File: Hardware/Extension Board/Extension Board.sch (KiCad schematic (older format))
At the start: 7 parts, among them J1 ARDUINO_DIGITAL, J2 ARDUINO_COMMS, J3 ARDUINO_ANALOG

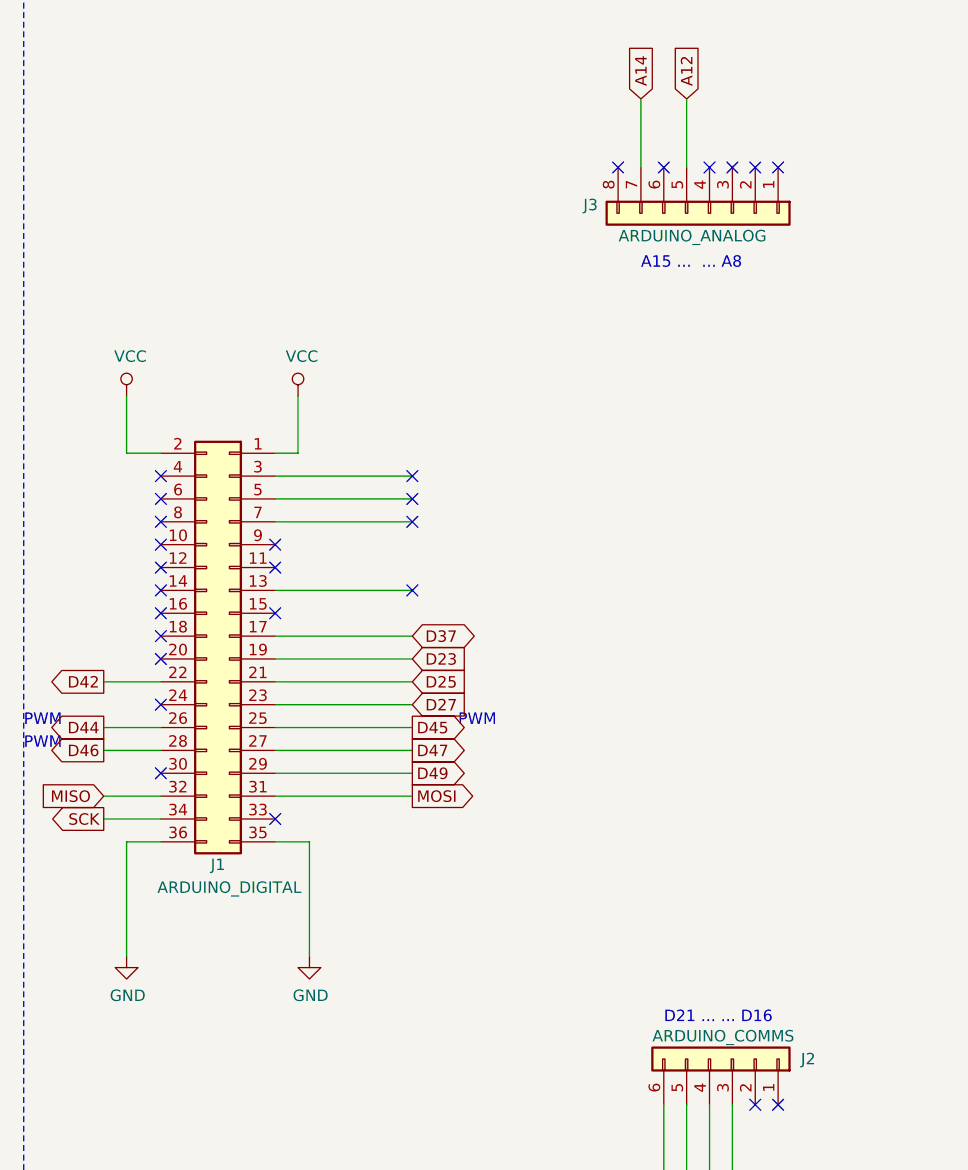
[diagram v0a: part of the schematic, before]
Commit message: début du routage
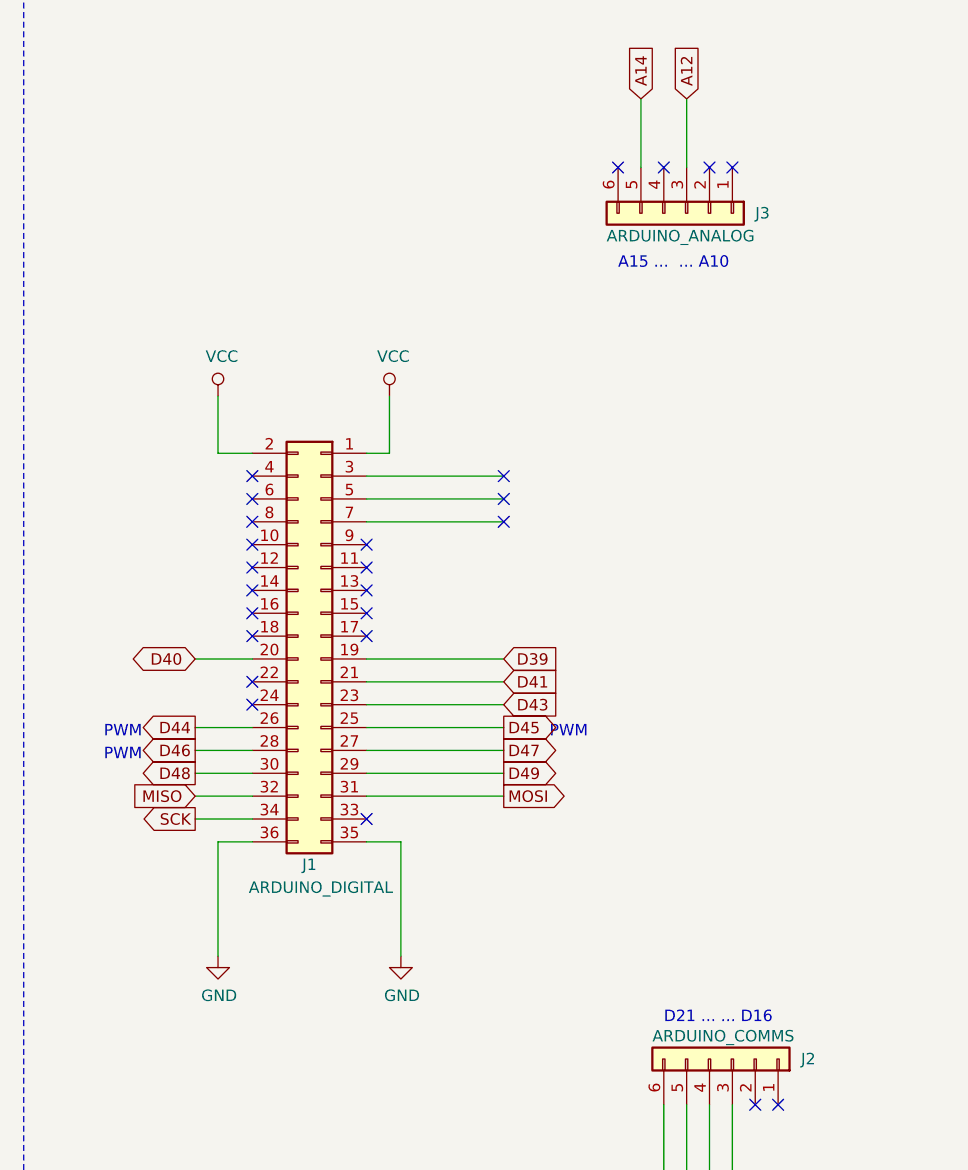
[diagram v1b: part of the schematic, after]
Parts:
- removed J3: ARDUINO_ANALOG, Connector_PinHeader_2.54mm:PinHeader_1x08_P2.54mm_Vertical, symbol Connector_Generic:Conn_01x08
- added J3: ARDUINO_ANALOG, Connector_PinHeader_2.54mm:PinHeader_1x06_P2.54mm_Vertical, symbol Connector_Generic:Conn_01x06
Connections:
- net A12: now also J3.3 (Pin_3)
- net A14: now also J3.5 (Pin_5)
- net D40: now reaches J1.20 (Pin_20)
- net D48: now reaches J1.30 (Pin_30)
- net D23 renamed D39
- net D25 renamed D41
- net D27 renamed D43
- net D37: no longer names the net of J1.17 (Pin_17)
- net D42: no longer names the net of J1.22 (Pin_22)
- no-connect marks 27 -> 25
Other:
- note added: "A15 ... ... A10"
- note removed: "A15 ... ... A8"
- moved on the sheet: J1
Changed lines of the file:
@@
 ARDUINO MEGA2560
-$Comp
-L Connector_Generic:Conn_01x08 J3
-U 1 1 5ED91F6A
-P 3700 1850
-F 0 "J3" V 3664 1362 50  0000 R CNN
-F 1 "ARDUINO_ANALOG" V 3800 2100 50  0000 R CNN
-F 2 "Connector_PinHeader_2.54mm:PinHeader_1x08_P2.54mm_Vertical" H 3700 1850 50  0001 C CNN
-F 3 "~" H 3700 1850 50  0001 C CNN
-	1    3700 1850
-	0    1    1    0
-$EndComp
-Wire Wire Line
-	1800 3500 2400 3500
 $Comp
 L power:VCC #PWR02
 U 1 1 5EDA4336
-P 1150 2650
-F 0 "#PWR02" H 1150 2500 50  0001 C CNN
-F 1 "VCC" H 1167 2823 50  0000 C CNN
-F 2 "" H 1150 2650 50  0001 C CNN
-F 3 "" H 1150 2650 50  0001 C CNN
-	1    1150 2650
+P 1550 2650
+F 0 "#PWR02" H 1550 2500 50  0001 C CNN
+F 1 "VCC" H 1567 2823 50  0000 C CNN
+F 2 "" H 1550 2650 50  0001 C CNN
+F 3 "" H 1550 2650 50  0001 C CNN
+	1    1550 2650
 	1    0    0    -1
 $EndComp
@@
 L power:GND #PWR01
 U 1 1 5EDAD0A2
-P 1150 5100
-F 0 "#PWR01" H 1150 4850 50  0001 C CNN
-F 1 "GND" H 1155 4927 50  0000 C CNN
-F 2 "" H 1150 5100 50  0001 C CNN
-F 3 "" H 1150 5100 50  0001 C CNN
-	1    1150 5100
+P 1550 5100
+F 0 "#PWR01" H 1550 4850 50  0001 C CNN
+F 1 "GND" H 1555 4927 50  0000 C CNN
+F 2 "" H 1550 5100 50  0001 C CNN
+F 3 "" H 1550 5100 50  0001 C CNN
+	1    1550 5100
 	1    0    0    -1
 $EndComp
@@
 Text GLabel 3600 6200 3    50   Output ~ 0
 SDA
-Text GLabel 2400 4400 2    50   Output ~ 0
+Text GLabel 2800 4400 2    50   Output ~ 0
 MOSI
-Text GLabel 1050 4400 0    50   Input ~ 0
+Text GLabel 1450 4400 0    50   Input ~ 0
 MISO
-Text GLabel 1050 4500 0    50   Output ~ 0
+Text GLabel 1450 4500 0    50   Output ~ 0
 SCK
 Wire Wire Line
-	1800 4400 2400 4400
-Wire Wire Line
-	1950 4600 1800 4600
+	2200 4400 2800 4400
+Wire Wire Line
+	2350 4600 2200 4600
 Text GLabel 3400 1350 1    50   Input ~ 0
 A14
@@
 Wire Wire Line
 	3600 1650 3600 1350
-Text GLabel 1050 3900 0    50   Output ~ 0
-D42
-Wire Wire Line
-	1800 3000 2400 3000
-Wire Wire Line
-	1800 3100 2400 3100
-Text GLabel 2400 4300 2    50   Output ~ 0
+Text GLabel 1450 4300 0    50   Output ~ 0
+D48
+Wire Wire Line
+	2200 3000 2800 3000
+Wire Wire Line
+	2200 3100 2800 3100
+Text GLabel 2800 4300 2    50   Output ~ 0
 D49
 Wire Wire Line
-	1800 3200 2400 3200
-NoConn ~ 1300 3200
-NoConn ~ 1300 3300
-NoConn ~ 1300 3400
-NoConn ~ 1800 4500
-Wire Wire Line
-	1900 2900 1800 2900
-NoConn ~ 1300 3000
-NoConn ~ 1300 3100
-NoConn ~ 4000 1650
-NoConn ~ 3900 1650
+	2200 3200 2800 3200
+NoConn ~ 1700 3200
+NoConn ~ 1700 3300
+NoConn ~ 1700 3400
+NoConn ~ 2200 4500
+Wire Wire Line
+	2300 2900 2200 2900
+NoConn ~ 1700 3000
+NoConn ~ 1700 3100
 NoConn ~ 3800 1650
 NoConn ~ 3700 1650
@@
 Wire Wire Line
 	3600 6200 3600 5750
-Text GLabel 1050 4100 0    50   Output ~ 0
+Text GLabel 1450 4100 0    50   Output ~ 0
 D44
-Text GLabel 1050 4200 0    50   Output ~ 0
+Text GLabel 1450 4200 0    50   Output ~ 0
 D46
-Text GLabel 2400 4000 2    50   Input ~ 0
-D27
-Text GLabel 2400 3900 2    50   Input ~ 0
-D25
-Text GLabel 2400 3800 2    50   Input ~ 0
-D23
+Text GLabel 2800 4000 2    50   Input ~ 0
+D43
+Text GLabel 2800 3900 2    50   Input ~ 0
+D41
+Text GLabel 2800 3800 2    50   Input ~ 0
+D39
 $Comp
 L Connector_Generic:Conn_01x06 J2
@@
 	1    0    0    -1
 $EndComp
-NoConn ~ 1300 4300
-NoConn ~ 1300 3700
-Wire Wire Line
-	1050 4100 1300 4100
-Wire Wire Line
-	1050 4200 1300 4200
-Wire Wire Line
-	1050 4400 1300 4400
-Wire Wire Line
-	1050 4500 1300 4500
-Wire Wire Line
-	1150 4600 1300 4600
-NoConn ~ 1300 3500
-Wire Wire Line
-	1150 2900 1300 2900
-NoConn ~ 1300 3600
-NoConn ~ 1800 3400
-Text Notes 3400 2100 0    50   ~ 0
-A15 ...  ... A8
+NoConn ~ 1700 3700
+Wire Wire Line
+	1450 4100 1700 4100
+Wire Wire Line
+	1450 4200 1700 4200
+Wire Wire Line
+	1450 4400 1700 4400
+Wire Wire Line
+	1450 4500 1700 4500
+Wire Wire Line
+	1550 4600 1700 4600
+NoConn ~ 1700 3500
+Wire Wire Line
+	1550 2900 1700 2900
+NoConn ~ 1700 3600
+NoConn ~ 2200 3400
+Text Notes 3300 2100 0    50   ~ 0
+A15 ...  ... A10
 Text Notes 3500 5400 0    50   ~ 0
 D21 ... ... D16
@@
 L power:GND #PWR0106
 U 1 1 6247305B
-P 1950 5100
-F 0 "#PWR0106" H 1950 4850 50  0001 C CNN
-F 1 "GND" H 1955 4927 50  0000 C CNN
-F 2 "" H 1950 5100 50  0001 C CNN
-F 3 "" H 1950 5100 50  0001 C CNN
-	1    1950 5100
-	1    0    0    -1
-$EndComp
-Wire Wire Line
-	1150 4600 1150 5100
-Wire Wire Line
-	1950 4600 1950 5100
+P 2350 5100
+F 0 "#PWR0106" H 2350 4850 50  0001 C CNN
+F 1 "GND" H 2355 4927 50  0000 C CNN
+F 2 "" H 2350 5100 50  0001 C CNN
+F 3 "" H 2350 5100 50  0001 C CNN
+	1    2350 5100
+	1    0    0    -1
+$EndComp
+Wire Wire Line
+	1550 4600 1550 5100
+Wire Wire Line
+	2350 4600 2350 5100
 $Comp
 L power:VCC #PWR0107
 U 1 1 6247ECAC
-P 1900 2650
-F 0 "#PWR0107" H 1900 2500 50  0001 C CNN
-F 1 "VCC" H 1917 2823 50  0000 C CNN
-F 2 "" H 1900 2650 50  0001 C CNN
-F 3 "" H 1900 2650 50  0001 C CNN
-	1    1900 2650
-	1    0    0    -1
-$EndComp
-Wire Wire Line
-	1900 2650 1900 2900
-Wire Wire Line
-	1150 2650 1150 2900
+P 2300 2650
+F 0 "#PWR0107" H 2300 2500 50  0001 C CNN
+F 1 "VCC" H 2317 2823 50  0000 C CNN
+F 2 "" H 2300 2650 50  0001 C CNN
+F 3 "" H 2300 2650 50  0001 C CNN
+	1    2300 2650
+	1    0    0    -1
+$EndComp
+Wire Wire Line
+	2300 2650 2300 2900
+Wire Wire Line
+	1550 2650 1550 2900
 Text GLabel 3800 6200 3    50   Input ~ 0
 D18
@@
 Wire Wire Line
 	3800 5750 3800 6200
-Text GLabel 2400 3700 2    50   BiDi ~ 0
-D37
-Wire Wire Line
-	1800 3700 2400 3700
+Text GLabel 1450 3800 0    50   BiDi ~ 0
+D40
 $Sheet
 S 5850 950  3650 800
@@
 F1 "Alimentation.sch" 50
 $EndSheet
-Text GLabel 2400 4100 2    50   Output ~ 0
+Text GLabel 2800 4100 2    50   Output ~ 0
 D45
 $Sheet
@@
 F1 "Audio.sch" 50
 $EndSheet
-NoConn ~ 1800 3300
-NoConn ~ 1300 3800
-NoConn ~ 1300 4000
+NoConn ~ 2200 3300
+NoConn ~ 1700 4000
 $Comp
 L Mechanical:MountingHole H3
@@
 	1    0    0    -1
 $EndComp
-NoConn ~ 1800 3600
-Wire Wire Line
-	1800 4200 2400 4200
-Wire Wire Line
-	2400 4300 1800 4300
-Wire Wire Line
-	2400 4100 1800 4100
+NoConn ~ 2200 3600
+Wire Wire Line
+	2200 4200 2800 4200
+Wire Wire Line
+	2800 4300 2200 4300
+Wire Wire Line
+	2800 4100 2200 4100
 $Comp
 L Connector_Generic:Conn_02x18_Odd_Even J1
 U 1 1 5ED8EC88
-P 1600 3700
-F 0 "J1" H 1650 2700 50  0000 C CNN
-F 1 "ARDUINO_DIGITAL" H 1600 2600 50  0000 C CNN
-F 2 "Connector_PinHeader_2.54mm:PinHeader_2x18_P2.54mm_Vertical" H 1600 3700 50  0001 C CNN
-F 3 "~" H 1600 3700 50  0001 C CNN
-	1    1600 3700
+P 2000 3700
+F 0 "J1" H 2050 2700 50  0000 C CNN
+F 1 "ARDUINO_DIGITAL" H 2000 2600 50  0000 C CNN
+F 2 "Connector_PinHeader_2.54mm:PinHeader_2x18_P2.54mm_Vertical" H 2000 3700 50  0001 C CNN
+F 3 "~" H 2000 3700 50  0001 C CNN
+	1    2000 3700
 	-1   0    0    -1
 $EndComp
-Text GLabel 2400 4200 2    50   Output ~ 0
+Text GLabel 2800 4200 2    50   Output ~ 0
 D47
-Text Notes 2600 4100 0    50   ~ 0
+Text Notes 3000 4150 0    50   ~ 0
 PWM
-Text Notes 700  4100 0    50   ~ 0
+Text Notes 1050 4150 0    50   ~ 0
 PWM\n
-Text Notes 700  4200 0    50   ~ 0
+Text Notes 1050 4250 0    50   ~ 0
 PWM
-Wire Wire Line
-	1050 3900 1300 3900
-NoConn ~ 2400 3500
-NoConn ~ 2400 3000
-NoConn ~ 2400 3100
-NoConn ~ 2400 3200
-Wire Wire Line
-	1800 3800 2400 3800
-Wire Wire Line
-	1800 3900 2400 3900
-Wire Wire Line
-	1800 4000 2400 4000
+NoConn ~ 2800 3000
+NoConn ~ 2800 3100
+NoConn ~ 2800 3200
+Wire Wire Line
+	2200 3800 2800 3800
+Wire Wire Line
+	2200 3900 2800 3900
+Wire Wire Line
+	2200 4000 2800 4000
+Wire Wire Line
+	1450 3800 1700 3800
+NoConn ~ 2200 3700
+NoConn ~ 2200 3500
+$Comp
+L Connector_Generic:Conn_01x06 J3
+U 1 1 6255C865
+P 3600 1850
+F 0 "J3" V 3600 2150 50  0000 L CNN
+F 1 "ARDUINO_ANALOG" V 3700 1500 50  0000 L CNN
+F 2 "Connector_PinHeader_2.54mm:PinHeader_1x06_P2.54mm_Vertical" H 3600 1850 50  0001 C CNN
+F 3 "~" H 3600 1850 50  0001 C CNN
+	1    3600 1850
+	0    1    1    0
+$EndComp
+Wire Wire Line
+	1700 4300 1450 4300
+NoConn ~ 1700 3900
 $EndSCHEMATC
